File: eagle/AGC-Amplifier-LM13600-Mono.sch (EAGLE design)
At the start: 11 parts, among them IC1 LM13600

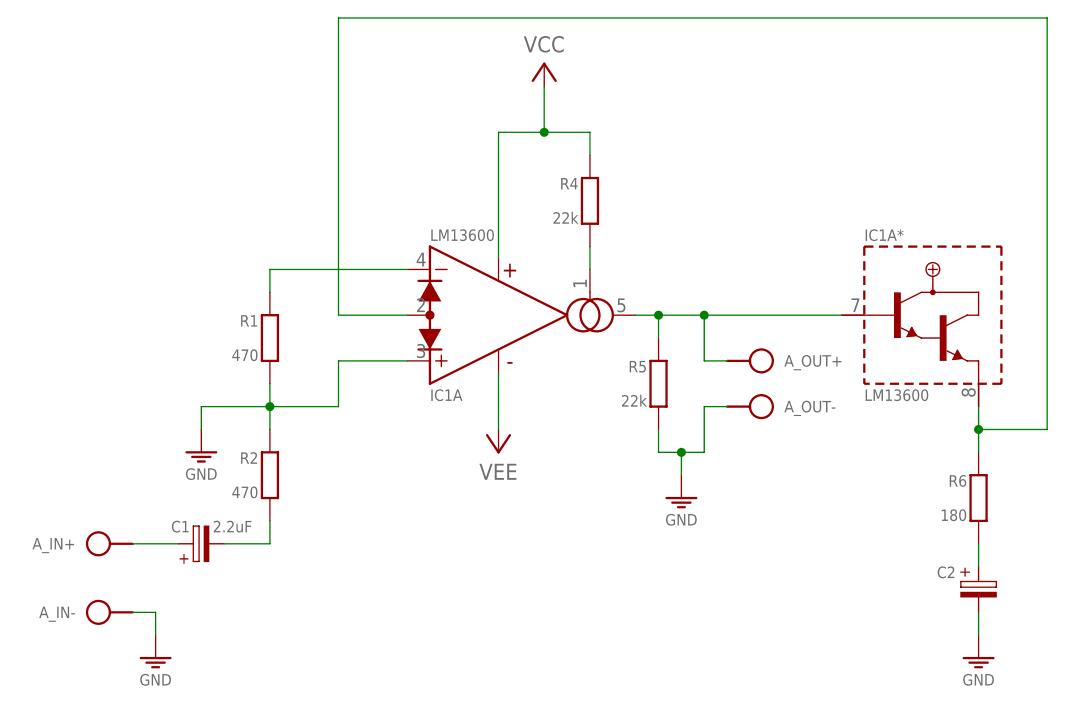
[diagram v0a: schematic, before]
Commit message: ...
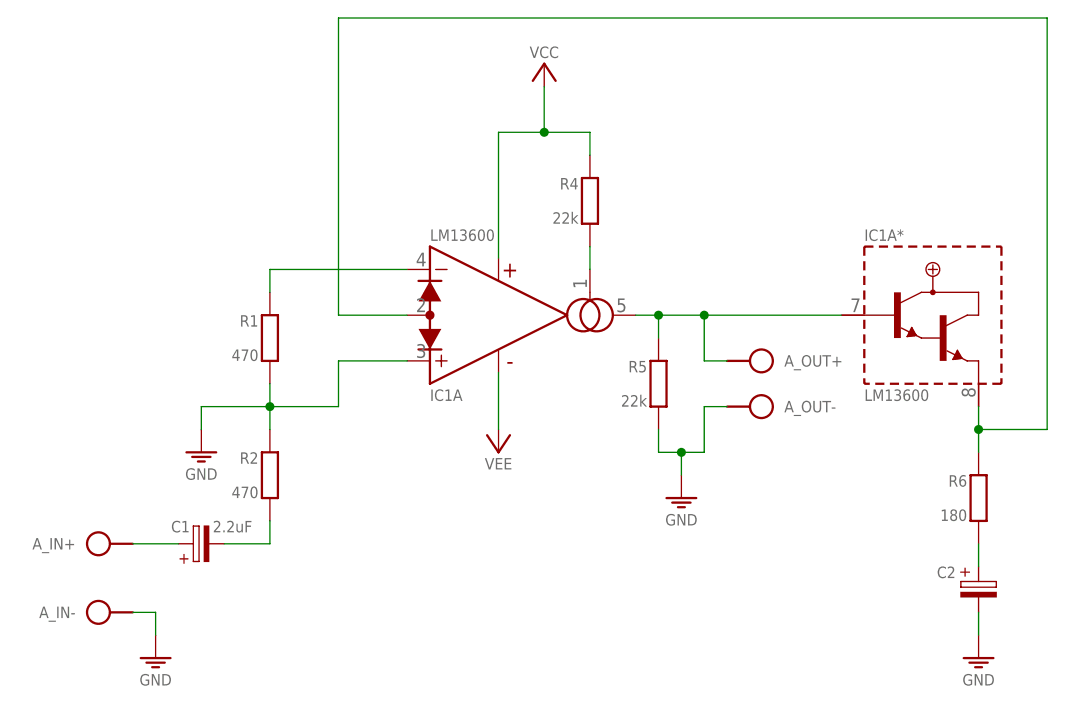
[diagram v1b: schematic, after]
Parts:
- removed U$3: VCC_GND_VEE, pad:VCC_GND_VEE
- added PWR: VCC_GND_VEEPWR-+GND-, pad:VCC_GND_VEEPWR-+GND-
- A_IN: value SPAD+--+ -> (none); device pad:SPAD+--+ -> pad:SPAD+-+-
- A_OUT: value SPAD+-+- -> (none)
- R1, R4, R6: device r:R0204/10-V -> r:R0202/7
- R5: device r:R0204/10-V -> r:R0202/7-V
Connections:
- net GND: now also PWRG$2.GND; no longer U$3G$2.GND
- net VCC: now also PWRG$1.VCC; no longer U$3G$1.VCC
- net VEE: now also PWRG$3.VEE; no longer U$3G$3.VEE
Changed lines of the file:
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@@
 </variantdefs>
 <classes>
-<class number="0" name="default" width="0" drill="0">
+<class number="0" name="default" width="0.6096" drill="0">
 </class>
 </classes>
 <parts>
 <part name="IC1" library="ic" deviceset="LM13600" device=""/>
-<part name="R4" library="r" deviceset="R" device="0204/10-V" value="22k"/>
-<part name="R5" library="r" deviceset="R" device="0204/10-V" value="22k"/>
-<part name="R1" library="r" deviceset="R" device="0204/10-V" value="470"/>
+<part name="R4" library="r" deviceset="R" device="0202/7" value="22k"/>
+<part name="R5" library="r" deviceset="R" device="0202/7-V" value="22k"/>
+<part name="R1" library="r" deviceset="R" device="0202/7" value="470"/>
 <part name="R2" library="r" deviceset="R" device="0204/10-V" value="470"/>
 <part name="C1" library="c" deviceset="CPOL-H" device="E2,5-4" value="2.2uF"/>
 <part name="C2" library="c" deviceset="CPOL" device="E2,5-4/V"/>
-<part name="R6" library="r" deviceset="R" device="0204/10-V" value="180"/>
+<part name="R6" library="r" deviceset="R" device="0202/7" value="180"/>
 <part name="S2" library="pad" deviceset="GND" device=""/>
 <part name="S3" library="pad" deviceset="GND" device=""/>
-<part name="U$3" library="pad" deviceset="VCC_GND_VEE" device=""/>
-<part name="A_IN" library="pad" deviceset="SPAD+-" device="-+"/>
+<part name="PWR" library="pad" deviceset="VCC_GND_VEE" device="PWR-+GND-" value="VCC_GND_VEEPWR-+GND-"/>
+<part name="A_IN" library="pad" deviceset="SPAD+-" device="+-"/>
 <part name="S1" library="pad" deviceset="GND" device=""/>
 <part name="A_OUT" library="pad" deviceset="SPAD+-" device="+-"/>
@@
 <instance part="S3" gate="1" x="60.96" y="35.56"/>
 <instance part="IC1" gate="G$5" x="40.64" y="55.88"/>
-<instance part="U$3" gate="G$1" x="45.72" y="81.28"/>
-<instance part="U$3" gate="G$2" x="7.62" y="43.18"/>
-<instance part="U$3" gate="G$3" x="40.64" y="43.18"/>
+<instance part="PWR" gate="G$1" x="45.72" y="81.28"/>
+<instance part="PWR" gate="G$2" x="7.62" y="43.18"/>
+<instance part="PWR" gate="G$3" x="40.64" y="43.18"/>
 <instance part="A_IN" gate="-" x="0" y="22.86"/>
 <instance part="A_IN" gate="+" x="0" y="30.48"/>
@@
 <wire x1="15.24" y1="45.72" x2="7.62" y2="45.72" width="0.1524" layer="91"/>
 <wire x1="7.62" y1="45.72" x2="7.62" y2="43.18" width="0.1524" layer="91"/>
-<pinref part="U$3" gate="G$2" pin="GND"/>
+<pinref part="PWR" gate="G$2" pin="GND"/>
 </segment>
 <segment>
@@
 <wire x1="40.64" y1="76.2" x2="45.72" y2="76.2" width="0.1524" layer="91"/>
 <junction x="45.72" y="76.2"/>
-<pinref part="U$3" gate="G$1" pin="VCC"/>
+<pinref part="PWR" gate="G$1" pin="VCC"/>
 </segment>
 </net>
@@
 <pinref part="IC1" gate="G$5" pin="V-"/>
 <wire x1="40.64" y1="43.18" x2="40.64" y2="49.53" width="0.1524" layer="91"/>
-<pinref part="U$3" gate="G$3" pin="VEE"/>
+<pinref part="PWR" gate="G$3" pin="VEE"/>
 </segment>
 </net>

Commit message: ...
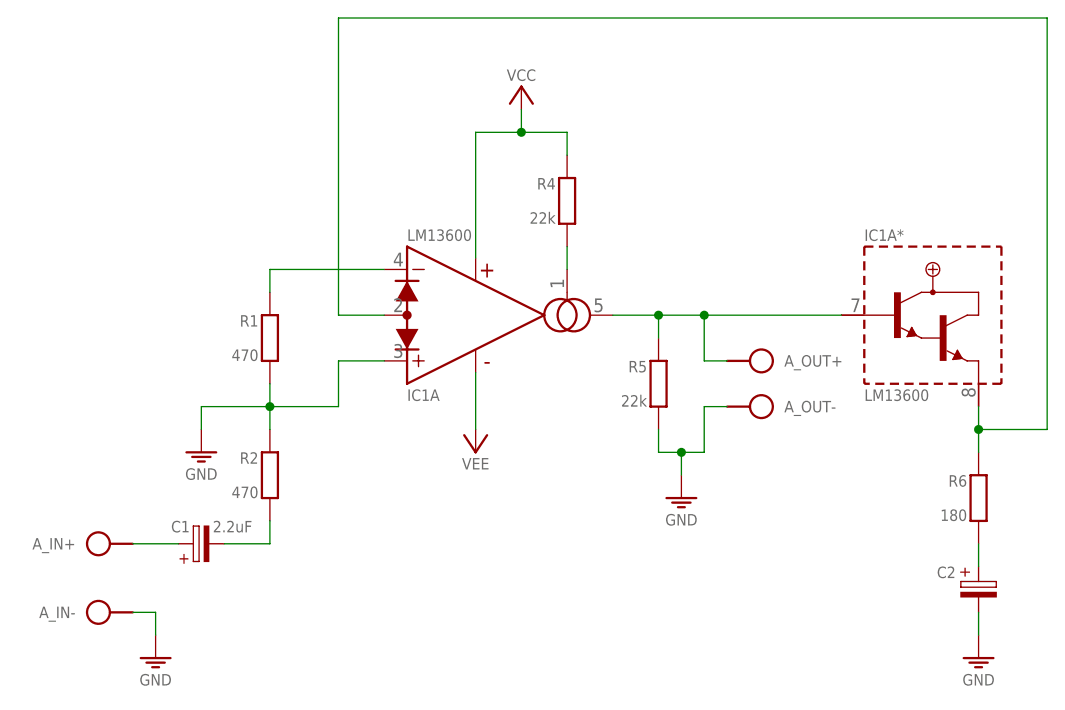
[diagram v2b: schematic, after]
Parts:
- R2: device r:R0204/10-V -> r:R0202/7-V
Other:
- moved on the sheet: IC1A, R4

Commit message: ...
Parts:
- C1: device c:CPOL-HE2,5-4 -> c:CPOL-HE2,5-4/V
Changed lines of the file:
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@@
 <part name="R1" library="r" deviceset="R" device="0202/7" value="470"/>
 <part name="R2" library="r" deviceset="R" device="0202/7-V" value="470"/>
-<part name="C1" library="c" deviceset="CPOL-H" device="E2,5-4" value="2.2uF"/>
+<part name="C1" library="c" deviceset="CPOL-H" device="E2,5-4/V" value="2.2uF"/>
 <part name="C2" library="c" deviceset="CPOL" device="E2,5-4/V"/>
 <part name="R6" library="r" deviceset="R" device="0202/7" value="180"/>
